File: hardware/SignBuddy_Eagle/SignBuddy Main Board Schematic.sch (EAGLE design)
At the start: 50 parts, among them U1 STM32L053C8T6D, U2 NCP115ASN330T2G

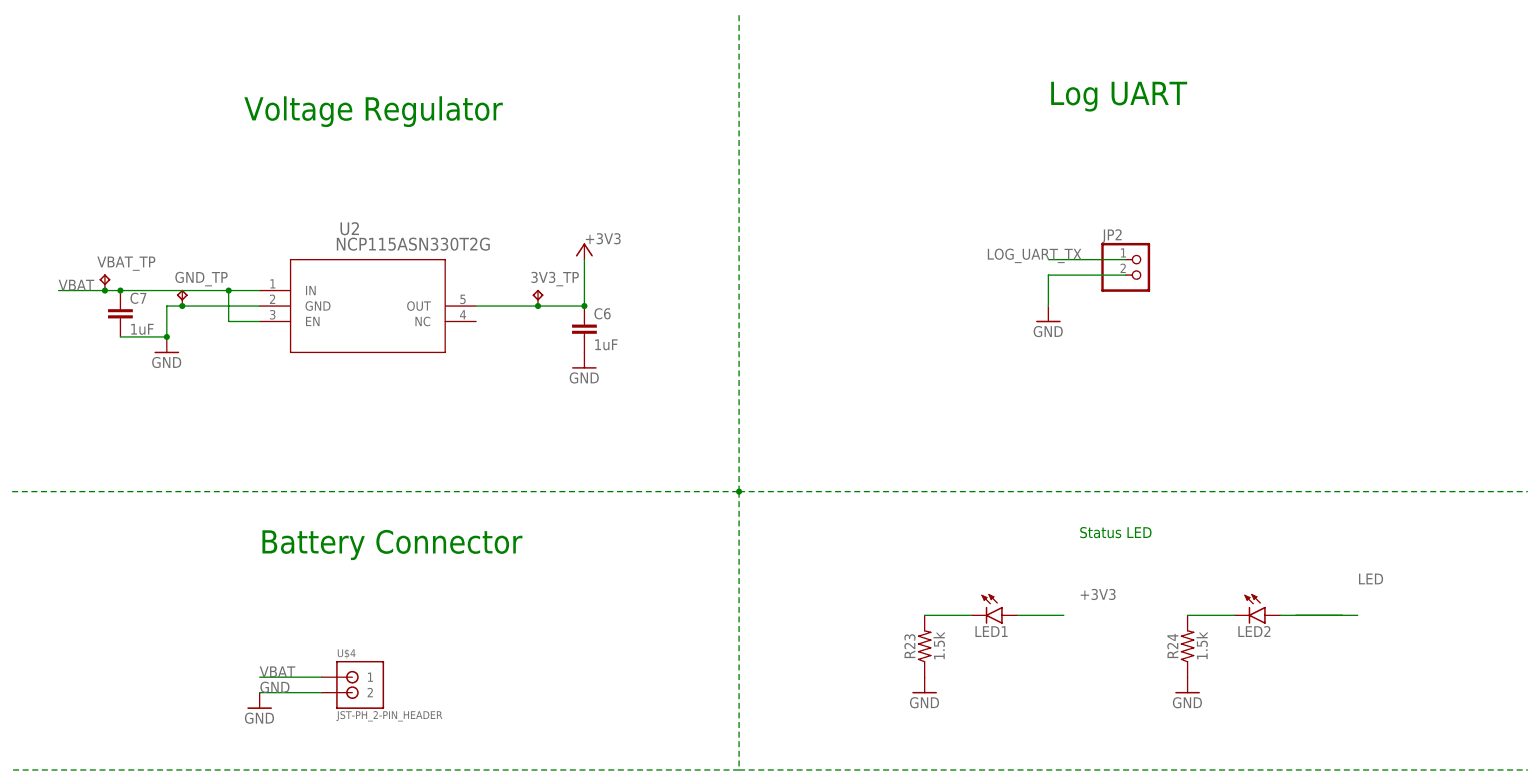
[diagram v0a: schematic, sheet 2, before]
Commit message: fixes
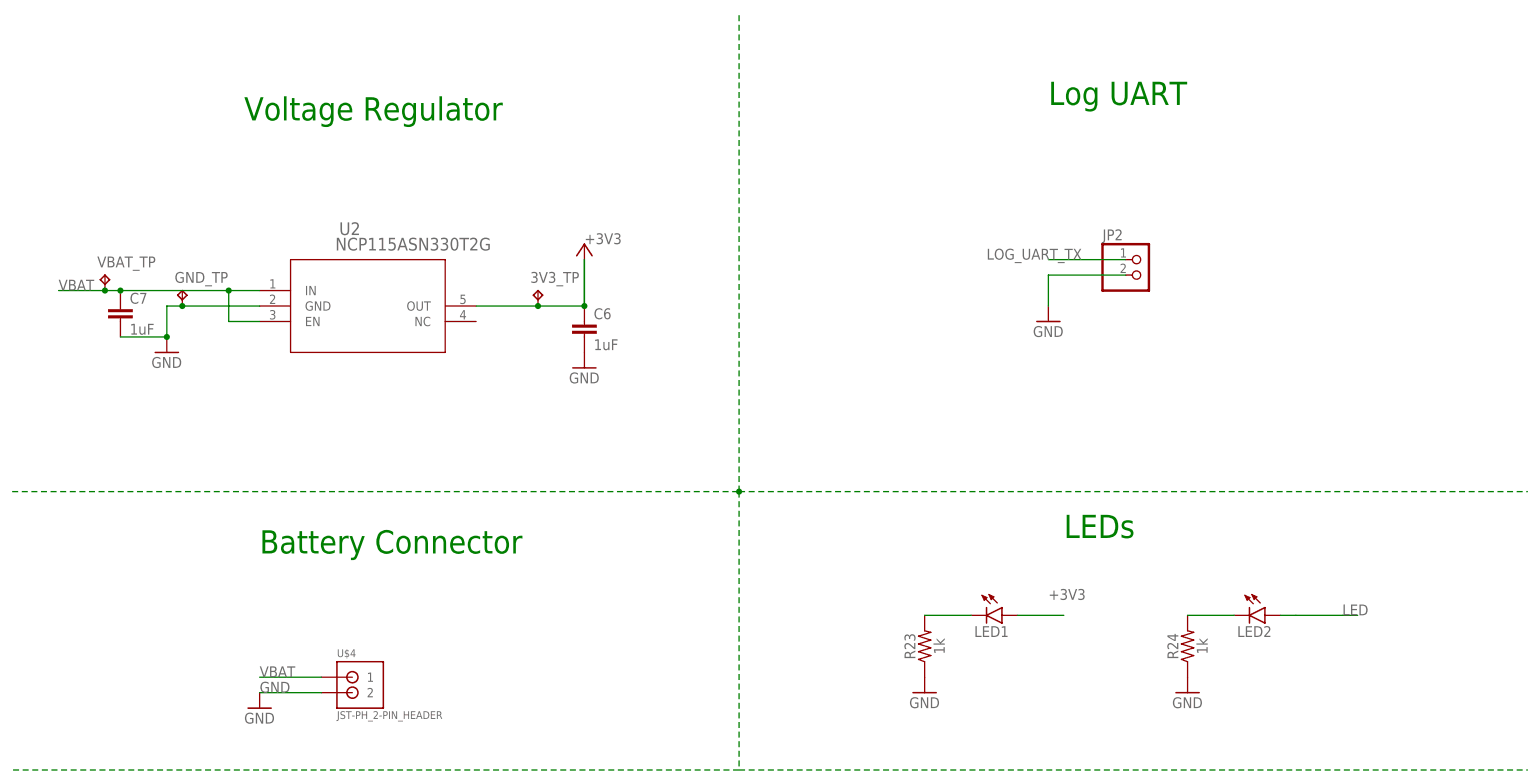
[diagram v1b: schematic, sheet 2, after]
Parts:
- R23, R24: value 1.5k -> 1k
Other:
- note added: "LEDs"
- note removed: "Status LED"
